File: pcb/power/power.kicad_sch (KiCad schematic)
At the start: 14 parts, among them J101 XT30PW-M, J102 Conn_02x10_Row_Letter_First

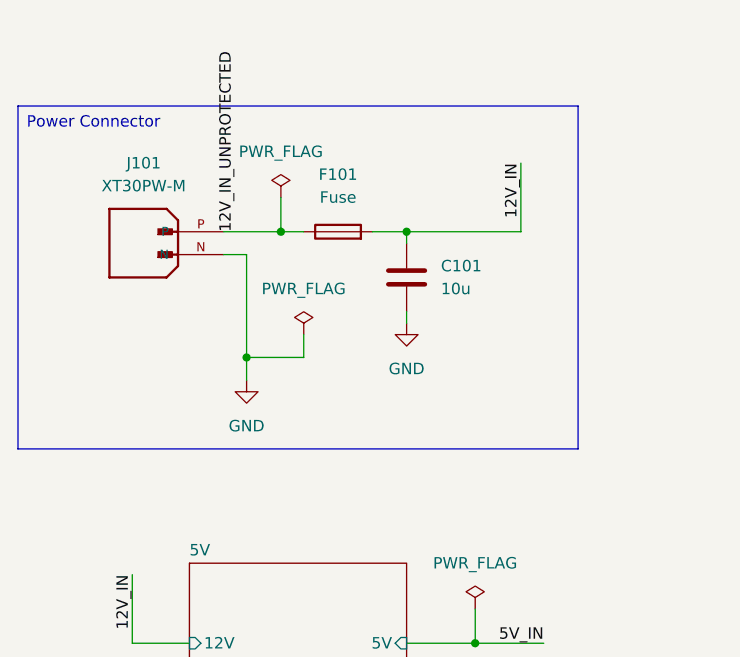
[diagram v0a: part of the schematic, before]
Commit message: update
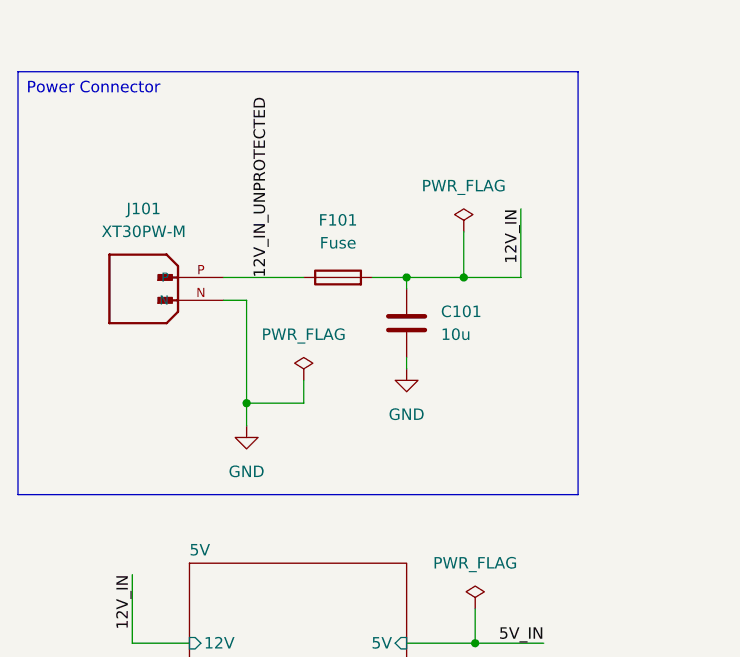
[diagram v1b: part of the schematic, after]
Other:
- moved on the sheet: C101, F101, J101
